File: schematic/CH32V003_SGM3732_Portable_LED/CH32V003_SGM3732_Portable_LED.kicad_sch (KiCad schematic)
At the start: 30 parts, among them J1 USB_C_Receptacle_USB2.0_16P, U1 CH32V003J4M6, U2 ME6211C33M5, U3 SGM3732

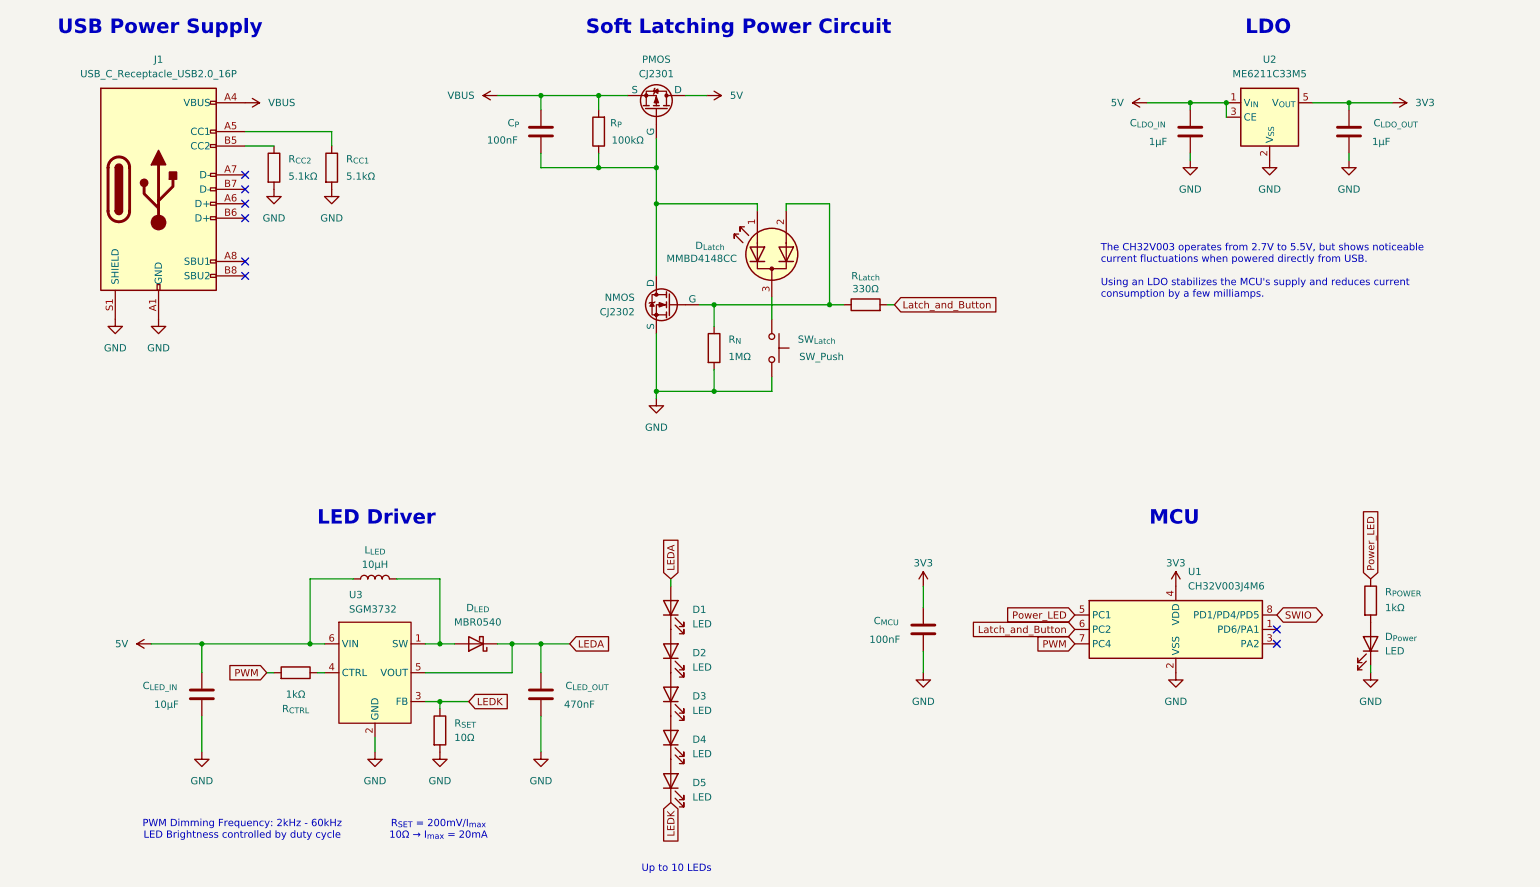
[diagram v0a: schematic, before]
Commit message: Update readme and schematic
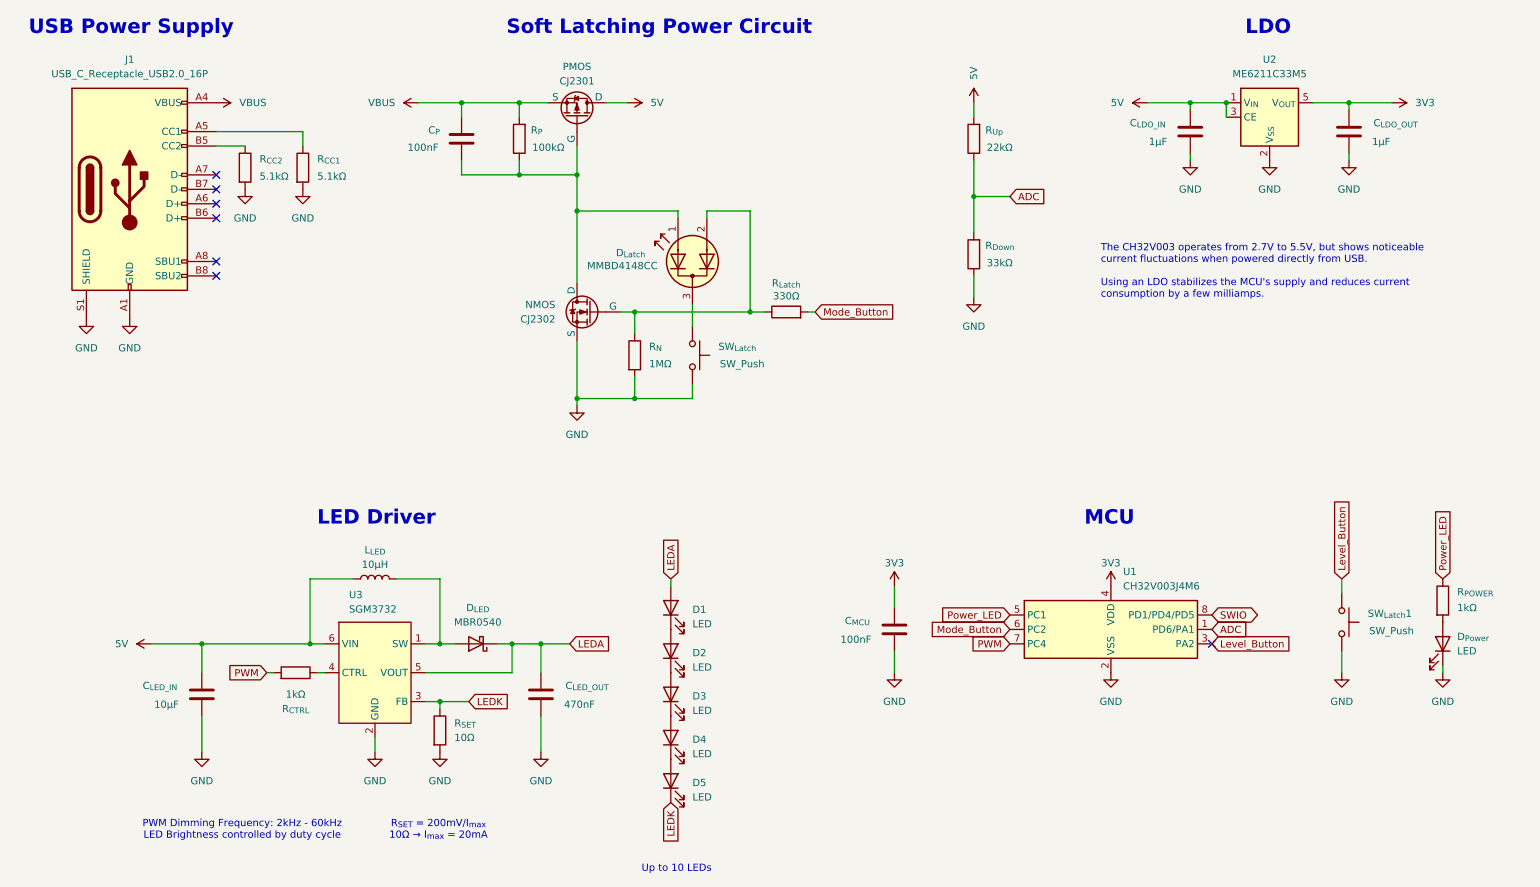
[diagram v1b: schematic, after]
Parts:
- added R_{Down}: 33kΩ, symbol Device:R
- added R_{Up}: 22kΩ, symbol Device:R
- added SW_{Latch}1: SW_Push, symbol Switch:SW_Push
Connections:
- net 5V: now also R_{Up}.2
- net GND: now also R_{Down}.1, SW_{Latch}1.1
- net ADC: now reaches U1.1 (PD6/PA1)
- net ADC: now also R_{Down}.2, R_{Up}.1
- net Level_Button: now reaches U1.3 (PA2)
- net Level_Button: now also SW_{Latch}1.2
- net Latch_and_Button renamed Mode_Button
- no-connect marks 8 -> 7
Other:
- moved on the sheet: C_{MCU}, C_{P}, D_{Latch}, D_{Power}, J1, NMOS, PMOS, R_{CC1}, R_{CC2}, R_{Latch}, R_{N}, R_{POWER}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
